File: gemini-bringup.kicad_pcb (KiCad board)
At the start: 4 copper layers, 187.2 x 112 mm, 282 parts, among them J1001 EXPANSION, J1101 SMBUS, J1201 SMBUS, J1301 SMBUS, J1401 IDC_BOX_HDR, J1501 I2CGPIO1, J1502 I2CGPIO0, J201 Conn_01x04, J202 Conn_ARM_JTAG_SWD_10, J203 Conn_2Rows-51Pins, J204 Conn_01x10, J301 Conn_ARM_JTAG_SWD_10, J302 HOST_UART, J303 AUX_HDR_J, J304 AUX_HDR_G, J401 RJ45_Würth_74980111211, J402 RJ45_Würth_74980111211, J501 SMBUS, J502 SMBUS, J503 SMBUS, J504 SMBUS, J601 Barrel_Jack, J701 FAN6, J702 FAN5, J703 FAN4, J704 FAN3, J705 FAN2, J706 FAN1, J801 IDC, J901 Micro_SD_Card, SW201 SW_SPDT, SW202 SW_SPST, SW301 RESET, SW302 BOOT0, U1101 TCA9802, U1201 TCA9802, U1301 TCA9802, U1401 TXB0106PWR, U1501 PCA9555PW, U301 STM32H753BITx, U302 MAX13235EET, U401 KSZ8863RLL, U501 LTC4306CGN, U601 OKI-78SR-3.3_1.5-W36-C, U602 INA219AxDCN, U603 INA219AxDCN, U701 MAX31790, U702 MCP1703A-5002_SOT89, U703 PCA9306DP1, U801 TXB0106PWR, U802 W25Q256FVFxx, U901 EMIF06-MSD02N16, Y301 8 MHz, Y302 32.768kHz, Y401 25MHz ±50ppm

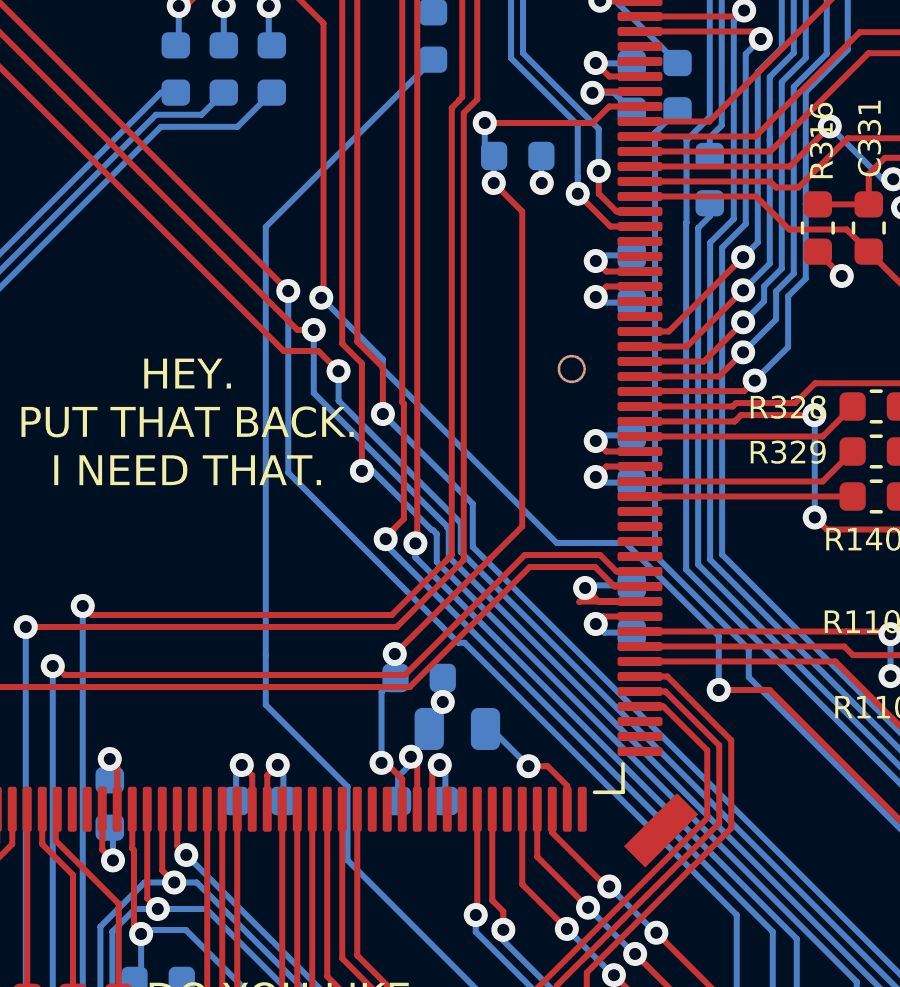
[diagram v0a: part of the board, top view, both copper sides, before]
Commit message: gemini-bringup: rework STM32H753 3.3V bypass caps in SW corner of footprint
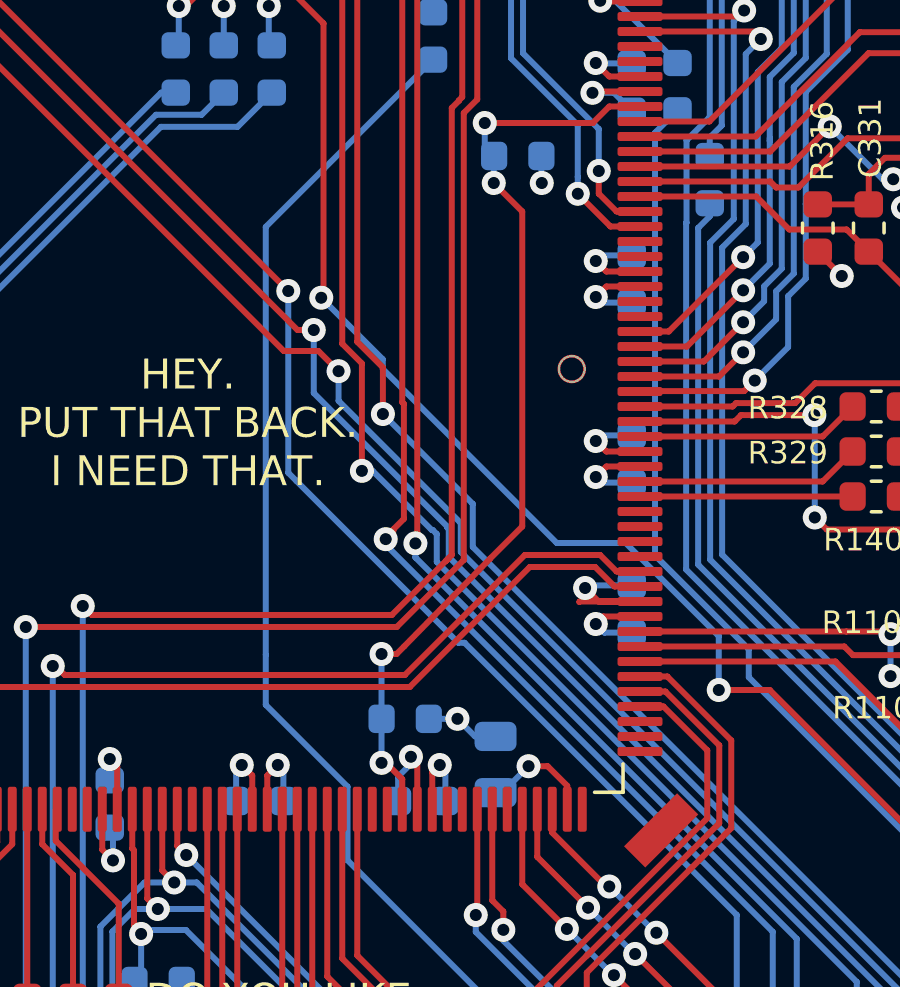
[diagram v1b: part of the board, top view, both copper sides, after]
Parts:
- moved C304 1.74 mm to (149.9, 83.2), turned to 90 degrees
- moved C302 1.44 mm to (146.8, 81.7)
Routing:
- net GND: track 338.0 -> 338.6 mm
- net +3V3: track 196.4 -> 195.8 mm
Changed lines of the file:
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@@
     (thickness 1.6)
     (drawings 58)
-    (tracks 4041)
+    (tracks 4040)
     (zones 0)
     (modules 282)
@@
   )
   (module Capacitor_SMD:C_0805_2012Metric (layer B.Cu)
-    (at 148.5875 82 180)
+    (at 149.86 83.185 90)
     (descr "Capacitor SMD 0805 (2012 Metric), square (rectangular) end terminal, IPC_7351 nominal, (Body size source: https://docs.google.com/spreadsheets/d/1BsfQQcO9C6DZCsRaXUlFlo91Tg2WpOkGARC1WS5S8t0/edit?usp=sharing), generated with kicad-footprint-generator")
     (tags capacitor)
     (attr smd)
-    (fp_text reference C304 (at 0 1.65) (layer B.SilkS)
+    (fp_text reference C304 (at 0 1.65 90) (layer B.SilkS)
       (effects (font (size 1 1) (thickness 0.15)) (justify mirror))
     )
-    (fp_text value 4.7uF (at 0 -1.65) (layer B.Fab)
+    (fp_text value 4.7uF (at 0 -1.65 90) (layer B.Fab)
       (effects (font (size 1 1) (thickness 0.15)) (justify mirror))
     )
@@
     (fp_line (start -1 0.6) (end 1 0.6) (layer B.Fab) (width 0.1))
     (fp_line (start -1 -0.6) (end -1 0.6) (layer B.Fab) (width 0.1))
-    (fp_text user %R (at 0 0) (layer B.Fab)
+    (fp_text user %R (at 0 0 90) (layer B.Fab)
       (effects (font (size 0.5 0.5) (thickness 0.08)) (justify mirror))
     )
-    (pad 2 smd roundrect (at 0.9375 0 180) (size 0.975 1.4) (layers B.Cu B.Paste B.Mask) (roundrect_rratio 0.25)
+    (pad 2 smd roundrect (at 0.9375 0 90) (size 0.975 1.4) (layers B.Cu B.Paste B.Mask) (roundrect_rratio 0.25)
       (net 1 GND))
-    (pad 1 smd roundrect (at -0.9375 0 180) (size 0.975 1.4) (layers B.Cu B.Paste B.Mask) (roundrect_rratio 0.25)
+    (pad 1 smd roundrect (at -0.9375 0 90) (size 0.975 1.4) (layers B.Cu B.Paste B.Mask) (roundrect_rratio 0.25)
       (net 6 +3V3))
     (model ${KISYS3DMOD}/Capacitor_SMD.3dshapes/C_0805_2012Metric.wrl
@@
   )
   (module Capacitor_SMD:C_0603_1608Metric (layer B.Cu)
-    (at 147.3125 80.3)
+    (at 146.847184 81.661)
     (descr "Capacitor SMD 0603 (1608 Metric), square (rectangular) end terminal, IPC_7351 nominal, (Body size source: http://www.tortai-tech.com/upload/download/2011102023233369053.pdf), generated with kicad-footprint-generator")
     (tags capacitor)
@@
   (via (at 147.03857 82.925306) (size 0.8) (drill 0.4) (layers F.Cu B.Cu) (net 1))
   (segment (start 147.25 83.136736) (end 147.03857 82.925306) (width 0.2) (layer F.Cu) (net 1))
-  (via (at 148.1 81.1) (size 0.8) (drill 0.4) (layers F.Cu B.Cu) (net 1))
-  (segment (start 148.1 80.3) (end 148.1 81.1) (width 0.2) (layer B.Cu) (net 1) (status 10))
   (segment (start 151.3875 62.9) (end 151.5 62.9) (width 0.2) (layer B.Cu) (net 1) (status 30))
   (via (at 137.107125 86.380496) (size 0.8) (drill 0.4) (layers F.Cu B.Cu) (net 1))
@@
   (segment (start 192.16 90.56) (end 192.2 90.6) (width 0.2) (layer F.Cu) (net 1))
   (segment (start 192.16 88.5) (end 192.16 90.56) (width 0.2) (layer F.Cu) (net 1))
-  (segment (start 147.8 81.4) (end 148.1 81.1) (width 0.2) (layer B.Cu) (net 1))
-  (segment (start 147.8 82) (end 147.8 81.4) (width 0.2) (layer B.Cu) (net 1))
   (via (at 185.8 84) (size 0.8) (drill 0.4) (layers F.Cu B.Cu) (net 1))
   (segment (start 184.64 84) (end 185.8 84) (width 0.2) (layer F.Cu) (net 1))
@@
   (segment (start 128.0335 80.5665) (end 128.397 80.5665) (width 0.2) (layer B.Cu) (net 1))
   (segment (start 126.8 81.8) (end 128.0335 80.5665) (width 0.2) (layer B.Cu) (net 1))
+  (via (at 148.59 81.661) (size 0.8) (drill 0.4) (layers F.Cu B.Cu) (net 1))
+  (segment (start 147.634684 81.661) (end 148.59 81.661) (width 0.2) (layer B.Cu) (net 1))
+  (segment (start 149.1765 82.2475) (end 148.59 81.661) (width 0.2) (layer B.Cu) (net 1))
+  (segment (start 149.86 82.2475) (end 149.1765 82.2475) (width 0.2) (layer B.Cu) (net 1))
   (segment (start 187.699901 21.699901) (end 182.3 16.3) (width 0.2) (layer F.Cu) (net 2))
   (segment (start 198.1 18.15) (end 194.550099 21.699901) (width 0.2) (layer F.Cu) (net 2))
@@
   (segment (start 65.35 28.6) (end 65.25 28.5) (width 0.2) (layer F.Cu) (net 4))
   (segment (start 69.8 28.6) (end 65.35 28.6) (width 0.2) (layer F.Cu) (net 4))
-  (via (at 146.5 79.5) (size 0.8) (drill 0.4) (layers F.Cu B.Cu) (net 5))
-  (segment (start 146.338669 79.661331) (end 146.5 79.5) (width 0.2) (layer F.Cu) (net 5))
+  (via (at 146.059684 79.5) (size 0.8) (drill 0.4) (layers F.Cu B.Cu) (net 5))
   (segment (start 146.75 83.67259) (end 146.338669 83.261259) (width 0.2) (layer F.Cu) (net 5))
   (segment (start 146.75 84.675) (end 146.75 83.67259) (width 0.2) (layer F.Cu) (net 5) (status 10))
-  (segment (start 146.5 80.275) (end 146.525 80.3) (width 0.2) (layer B.Cu) (net 5) (status 30))
-  (segment (start 146.5 79.5) (end 146.5 80.275) (width 0.2) (layer B.Cu) (net 5) (status 20))
   (via (at 149.8 63.8) (size 0.8) (drill 0.4) (layers F.Cu B.Cu) (net 5))
   (segment (start 149.8 62.9125) (end 149.8125 62.9) (width 0.2) (layer B.Cu) (net 5) (status 30))
@@
   (segment (start 146.191712 83.261259) (end 146.059684 83.129231) (width 0.2) (layer F.Cu) (net 5))
   (segment (start 146.338669 83.261259) (end 146.191712 83.261259) (width 0.2) (layer F.Cu) (net 5))
-  (segment (start 146.059684 80.765316) (end 146.525 80.3) (width 0.2) (layer B.Cu) (net 5) (status 20))
-  (segment (start 146.059684 83.129231) (end 146.059684 80.765316) (width 0.2) (layer B.Cu) (net 5))
   (via (at 149.5 61.8) (size 0.8) (drill 0.4) (layers F.Cu B.Cu) (net 5))
   (segment (start 149.5 62.5875) (end 149.8125 62.9) (width 0.2) (layer B.Cu) (net 5) (status 30))
@@
   (segment (start 153.1 61.8) (end 149.5 61.8) (width 0.2) (layer F.Cu) (net 5))
   (segment (start 153.65 61.25) (end 153.1 61.8) (width 0.2) (layer F.Cu) (net 5))
-  (segment (start 149.8 63.8) (end 150.75 64.75) (width 0.2) (layer F.Cu) (net 5))
-  (segment (start 150.75 75.25) (end 149.675 76.325) (width 0.2) (layer F.Cu) (net 5))
-  (segment (start 150.75 64.75) (end 150.75 75.25) (width 0.2) (layer F.Cu) (net 5))
-  (segment (start 146.5 79.5) (end 149.675 76.325) (width 0.2) (layer F.Cu) (net 5))
+  (segment (start 150.75 64.75) (end 149.8 63.8) (width 0.2) (layer F.Cu) (net 5))
+  (segment (start 150.75 75.25) (end 150.75 64.75) (width 0.2) (layer F.Cu) (net 5))
+  (segment (start 149.675 76.325) (end 150.75 75.25) (width 0.2) (layer F.Cu) (net 5))
+  (segment (start 146.812 79.248) (end 149.675 76.325) (width 0.2) (layer F.Cu) (net 5))
+  (segment (start 146.56 79.5) (end 146.812 79.248) (width 0.2) (layer F.Cu) (net 5))
+  (segment (start 146.059684 79.5) (end 146.56 79.5) (width 0.2) (layer F.Cu) (net 5))
+  (segment (start 146.059684 81.661) (end 146.059684 79.5) (width 0.2) (layer B.Cu) (net 5))
+  (segment (start 146.059684 83.129231) (end 146.059684 81.661) (width 0.2) (layer B.Cu) (net 5))
   (segment (start 208.8025 35.8625) (end 208.99 36.05) (width 0.3) (layer F.Cu) (net 6) (status 30))
   (segment (start 207.3 35.8625) (end 208.8025 35.8625) (width 0.3) (layer F.Cu) (net 6) (status 30))
@@
   (segment (start 182.2125 102.7875) (end 182.2 102.8) (width 0.2) (layer F.Cu) (net 6))
   (segment (start 182.2125 101.8) (end 182.2125 102.7875) (width 0.2) (layer F.Cu) (net 6))
-  (segment (start 149.72038 82) (end 149.375 82) (width 0.2) (layer B.Cu) (net 6))
-  (segment (start 150.96019 83.23981) (end 149.72038 82) (width 0.2) (layer B.Cu) (net 6))
   (via (at 178.4 115.2) (size 0.8) (drill 0.4) (layers F.Cu B.Cu) (net 6))
   (segment (start 177.575 115.2) (end 178.4 115.2) (width 0.2) (layer F.Cu) (net 6))
@@
   (via (at 59.584 37.986) (size 0.8) (drill 0.4) (layers F.Cu B.Cu) (net 6))
   (segment (start 60.734 37.986) (end 59.584 37.986) (width 0.4) (layer F.Cu) (net 6))
+  (segment (start 150.0775 84.1225) (end 150.96019 83.23981) (width 0.2) (layer B.Cu) (net 6))
+  (segment (start 149.86 84.1225) (end 150.0775 84.1225) (width 0.2) (layer B.Cu) (net 6))
   (segment (start 119.714 73.25) (end 119.304 73.66) (width 0.2) (layer F.Cu) (net 7))
   (segment (start 125.325 73.25) (end 119.714 73.25) (width 0.2) (layer F.Cu) (net 7))

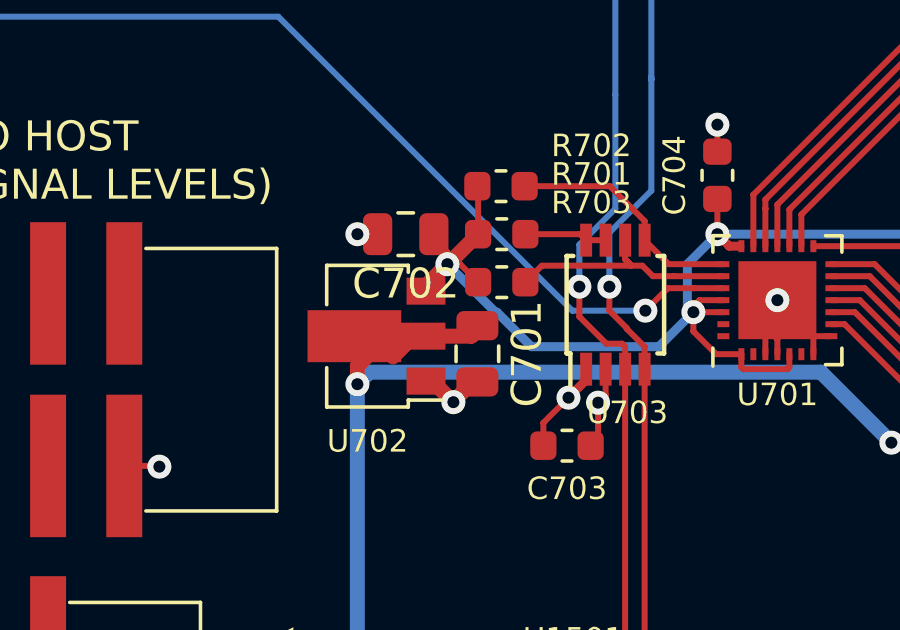
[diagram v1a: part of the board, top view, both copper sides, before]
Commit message: gemini-bringup: rework FAN5V bypass caps
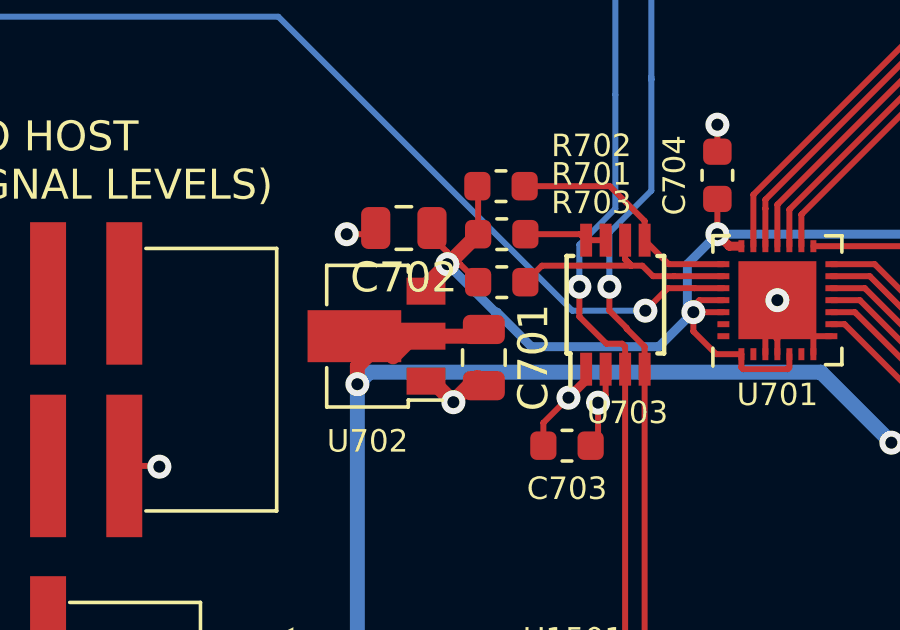
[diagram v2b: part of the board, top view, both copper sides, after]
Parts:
- moved C701 0.25 mm to (204.2, 59.6)
- moved C702 0.21 mm to (201.5, 55.2)
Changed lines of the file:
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@@
     (37 F.SilkS user)
     (38 B.Mask user hide)
-    (39 F.Mask user)
+    (39 F.Mask user hide)
     (40 Dwgs.User user hide)
     (41 Cmts.User user hide)
@@
   )
   (module Capacitor_SMD:C_0805_2012Metric (layer F.Cu)
-    (at 201.6125 55.45 180)
+    (at 201.549 55.245 180)
     (descr "Capacitor SMD 0805 (2012 Metric), square (rectangular) end terminal, IPC_7351 nominal, (Body size source: https://docs.google.com/spreadsheets/d/1BsfQQcO9C6DZCsRaXUlFlo91Tg2WpOkGARC1WS5S8t0/edit?usp=sharing), generated with kicad-footprint-generator")
     (tags capacitor)
@@
   )
   (module Capacitor_SMD:C_0805_2012Metric (layer F.Cu)
-    (at 204 59.4375 270)
+    (at 204.216 59.563 270)
     (descr "Capacitor SMD 0805 (2012 Metric), square (rectangular) end terminal, IPC_7351 nominal, (Body size source: https://docs.google.com/spreadsheets/d/1BsfQQcO9C6DZCsRaXUlFlo91Tg2WpOkGARC1WS5S8t0/edit?usp=sharing), generated with kicad-footprint-generator")
     (tags capacitor)
@@
   (segment (start 215.2 58.85) (end 214.65 58.3) (width 0.2) (layer F.Cu) (net 1) (status 30))
   (segment (start 215.8 58.85) (end 215.2 58.85) (width 0.2) (layer F.Cu) (net 1) (status 30))
-  (via (at 200 55.45) (size 0.8) (drill 0.4) (layers F.Cu B.Cu) (net 1))
-  (segment (start 200.825 55.45) (end 200 55.45) (width 0.2) (layer F.Cu) (net 1) (status 10))
   (via (at 203.2 61.05) (size 0.8) (drill 0.4) (layers F.Cu B.Cu) (net 1))
   (segment (start 202.5 60.35) (end 203.2 61.05) (width 0.5) (layer F.Cu) (net 1) (status 10))
@@
   (segment (start 149.1765 82.2475) (end 148.59 81.661) (width 0.2) (layer B.Cu) (net 1))
   (segment (start 149.86 82.2475) (end 149.1765 82.2475) (width 0.2) (layer B.Cu) (net 1))
+  (via (at 199.644 55.45) (size 0.8) (drill 0.4) (layers F.Cu B.Cu) (net 1))
+  (segment (start 200.825 55.45) (end 199.644 55.45) (width 0.2) (layer F.Cu) (net 1))
   (segment (start 187.699901 21.699901) (end 182.3 16.3) (width 0.2) (layer F.Cu) (net 2))
   (segment (start 198.1 18.15) (end 194.550099 21.699901) (width 0.2) (layer F.Cu) (net 2))
